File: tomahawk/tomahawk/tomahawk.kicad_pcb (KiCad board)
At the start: 2 copper layers, 79 parts, among them SW1 SW_Push, SW10 SW_Push, SW11 SW_Push, SW12 SW_Push, SW13 SW_Push, SW14 SW_Push, SW15 SW_Push, SW16 SW_Push, SW17 SW_Push, SW18 SW_Push, SW19 SW_Push, SW2 SW_Push, SW20 SW_Push, SW21 SW_Push, SW22 SW_Push, SW23 SW_Push, SW24 SW_Push, SW25 SW_Push, SW26 SW_Push, SW27 SW_Push, SW28 SW_Push, SW29 SW_Push, SW3 SW_Push, SW30 SW_Push, SW31 SW_Push, SW32 SW_Push, SW33 SW_Push, SW34 SW_Push, SW35 SW_Push, SW36 SW_Push, SW37 SW_Push, SW38 SW_Push, SW39 SW_Push, SW4 SW_Push, SW5 SW_Push, SW6 SW_Push, SW7 SW_Push, SW8 SW_Push, SW9 SW_Push

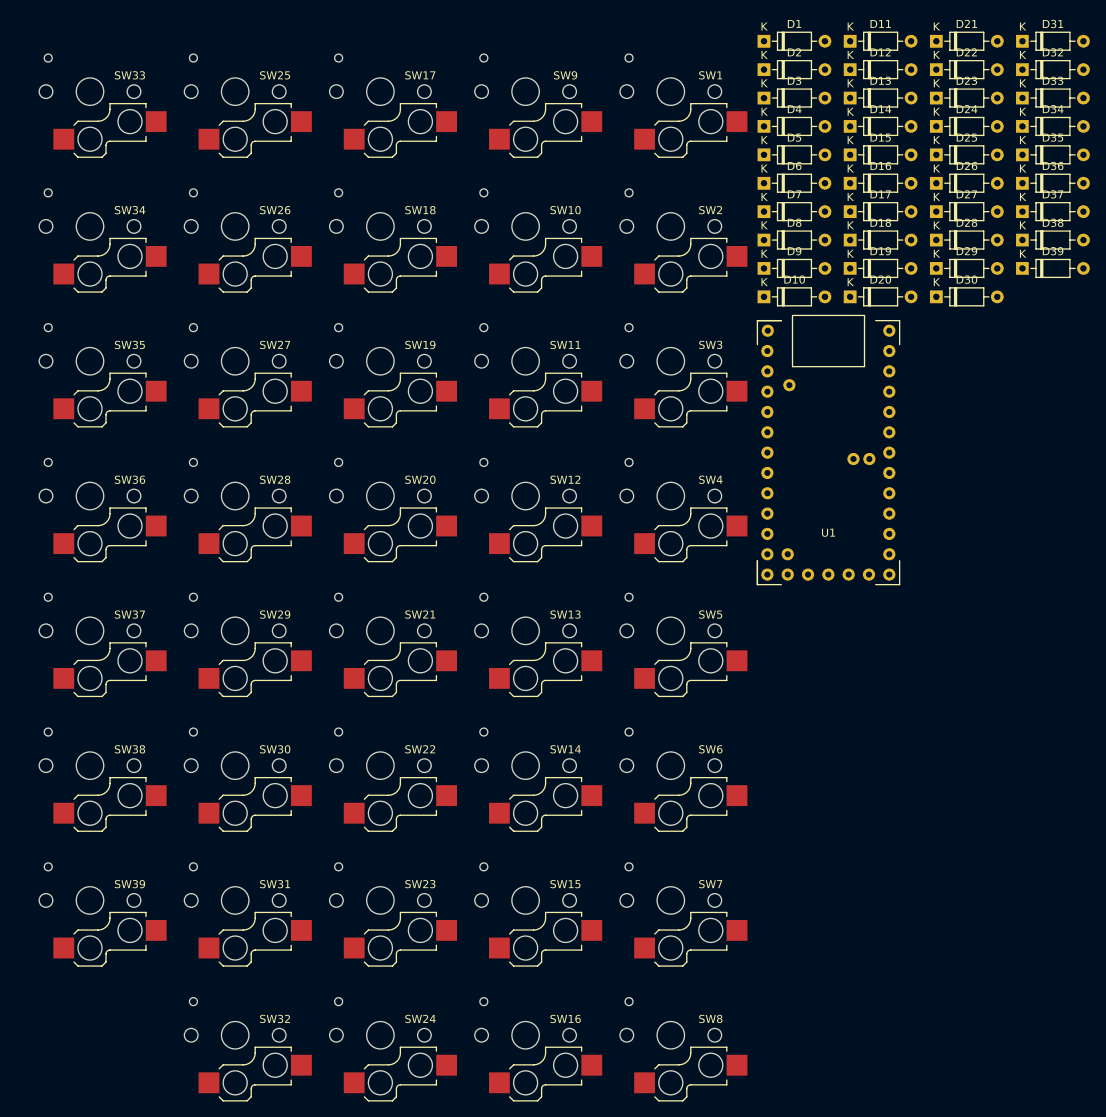
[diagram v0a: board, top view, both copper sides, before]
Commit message: updated footprints and pcb
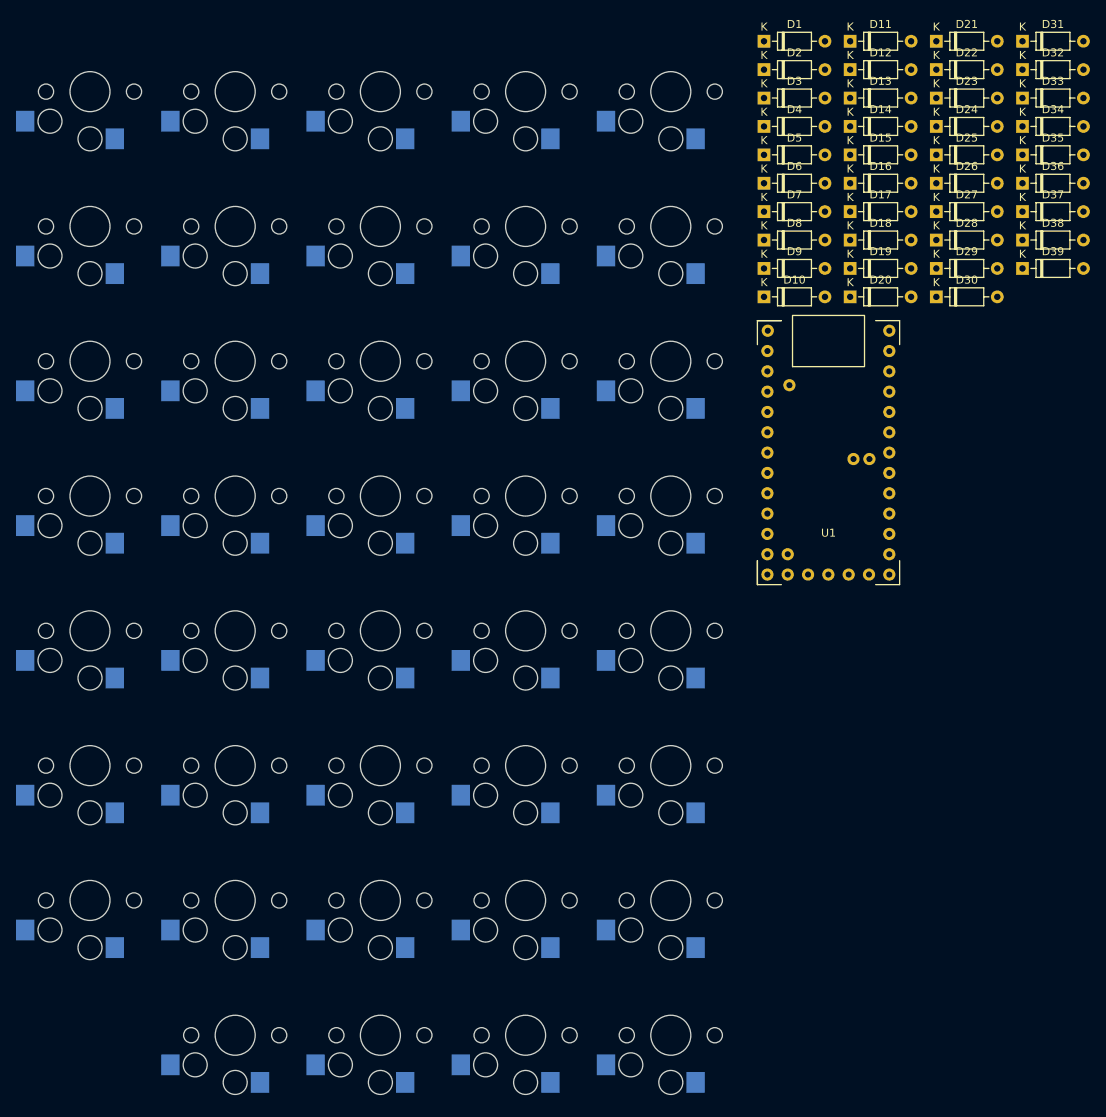
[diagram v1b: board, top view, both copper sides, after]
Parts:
- SW1, SW10, SW11, SW12, SW13, SW14, SW15, SW16, SW17, SW18, SW19, SW2, SW20, SW21, SW22, SW23, SW24, SW25, SW26, SW27, SW28, SW29, SW3, SW30, SW31, SW32, SW33, SW34, SW35, SW36, SW37, SW38, SW39, SW4, SW5, SW6, SW7, SW8, SW9: footprint Keyswitches:Kailh_socket_PG1350 -> Foostan:keyswitch_choc12_hotswap_1u
- U1: footprint ProMicro_RP2040:pro_micro_rp2040 -> ProMicro RP2040:pro_micro_rp2040
